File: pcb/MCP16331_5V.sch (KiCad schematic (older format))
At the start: 12 parts, among them U8 MCP16331T

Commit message: Fix inductor (old one was no longer available)
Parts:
- L4: footprint Inductors_local:Inductor_Würth_SPC_4818 -> Inductors_local:Inductor_Würth_WE-PD2_4532
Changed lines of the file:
@@
 F 0 "L4" V 6590 3450 50  0000 C CNN
 F 1 "22µ" V 6499 3450 50  0000 C CNN
-F 2 "Inductors_local:Inductor_Würth_SPC_4818" V 6498 3450 50  0001 C CNN
+F 2 "Inductors_local:Inductor_Würth_WE-PD2_4532" V 6498 3450 50  0001 C CNN
 F 3 "http://katalog.we-online.de/pbs/datasheet/744773122.pdf" V 6498 3450 50  0001 C CNN
 F 4 "732-1258-1-ND" H 6400 3450 60  0001 C CNN "Digi-Key Part Number"

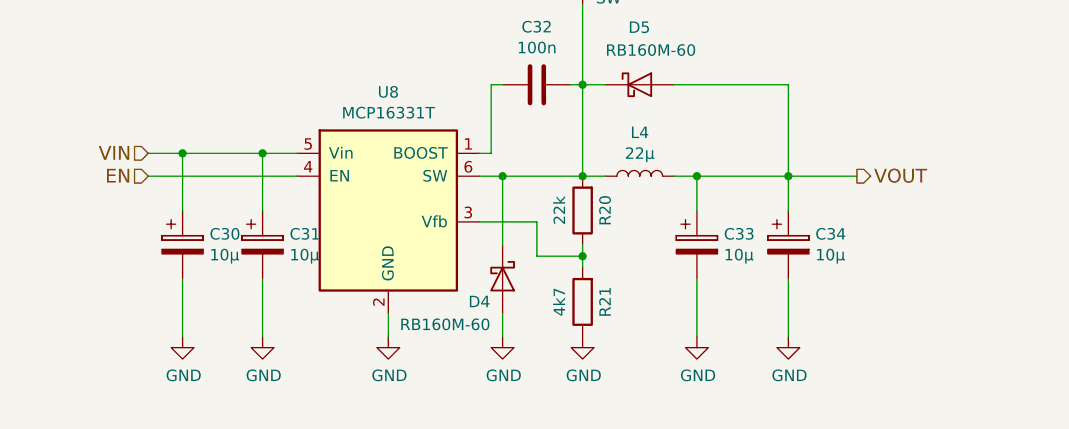
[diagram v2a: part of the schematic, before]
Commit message: Add some improvements, fix issue with schematic error
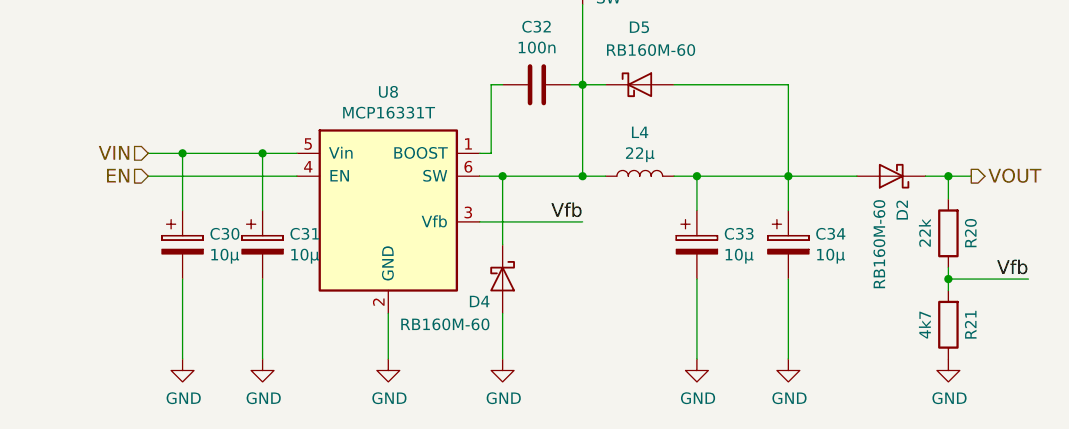
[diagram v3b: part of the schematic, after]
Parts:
- added D2: RB160M-60, Diodes_SMD:SOD-123, symbol D_Schottky
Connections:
- net VOUT: now also R20.2, D2.1 (K); no longer C33.1, C34.1, D5.2 (A), L4.2
- net Vfb: now reaches R20.1, R21.2, U8.3 (Vfb)
- net at C32.2, D4.1 (K), D5.1 (K)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: no longer R20.2
- new net: C33.1, C34.1, D2.2 (A), D5.2 (A), L4.2
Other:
- moved on the sheet: R20, R21
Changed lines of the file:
@@
 LIBS:a4955glptr-t
 LIBS:ap2112k-3.3trg1
+LIBS:lm75bd
+LIBS:mechanical
 LIBS:HighPower-Mechaduino-cache
 EELAYER 25 0
@@
 $EndComp
 $Comp
-L GND #PWR088
+L GND #PWR092
 U 1 1 580BA37A
-P 5300 4150
-F 0 "#PWR088" H 5300 3900 50  0001 C CNN
-F 1 "GND" H 5305 3977 50  0000 C CNN
-F 2 "" H 5300 4150 50  0000 C CNN
-F 3 "" H 5300 4150 50  0000 C CNN
-	1    5300 4150
-	1    0    0    -1
-$EndComp
-Wire Wire Line
-	5300 4050 5300 4150
+P 5300 4250
+F 0 "#PWR092" H 5300 4000 50  0001 C CNN
+F 1 "GND" H 5305 4077 50  0000 C CNN
+F 2 "" H 5300 4250 50  0000 C CNN
+F 3 "" H 5300 4250 50  0000 C CNN
+	1    5300 4250
+	1    0    0    -1
+$EndComp
+Wire Wire Line
+	5300 4050 5300 4250
 $Comp
 L CP C31
@@
 $EndComp
 $Comp
-L GND #PWR089
+L GND #PWR093
 U 1 1 580BA3A1
-P 4750 4150
-F 0 "#PWR089" H 4750 3900 50  0001 C CNN
-F 1 "GND" H 4755 3977 50  0000 C CNN
-F 2 "" H 4750 4150 50  0000 C CNN
-F 3 "" H 4750 4150 50  0000 C CNN
-	1    4750 4150
-	1    0    0    -1
-$EndComp
-$Comp
-L GND #PWR090
+P 4750 4250
+F 0 "#PWR093" H 4750 4000 50  0001 C CNN
+F 1 "GND" H 4755 4077 50  0000 C CNN
+F 2 "" H 4750 4250 50  0000 C CNN
+F 3 "" H 4750 4250 50  0000 C CNN
+	1    4750 4250
+	1    0    0    -1
+$EndComp
+$Comp
+L GND #PWR094
 U 1 1 580BA3A7
-P 4400 4150
-F 0 "#PWR090" H 4400 3900 50  0001 C CNN
-F 1 "GND" H 4405 3977 50  0000 C CNN
-F 2 "" H 4400 4150 50  0000 C CNN
-F 3 "" H 4400 4150 50  0000 C CNN
-	1    4400 4150
-	1    0    0    -1
-$EndComp
-Wire Wire Line
-	4750 3900 4750 4150
-Wire Wire Line
-	4400 3900 4400 4150
+P 4400 4250
+F 0 "#PWR094" H 4400 4000 50  0001 C CNN
+F 1 "GND" H 4405 4077 50  0000 C CNN
+F 2 "" H 4400 4250 50  0000 C CNN
+F 3 "" H 4400 4250 50  0000 C CNN
+	1    4400 4250
+	1    0    0    -1
+$EndComp
+Wire Wire Line
+	4750 3900 4750 4250
+Wire Wire Line
+	4400 3900 4400 4250
 $Comp
 L C C32
@@
 $EndComp
 $Comp
-L GND #PWR091
+L GND #PWR095
 U 1 1 580BA3CF
-P 6650 4150
-F 0 "#PWR091" H 6650 3900 50  0001 C CNN
-F 1 "GND" H 6655 3977 50  0000 C CNN
-F 2 "" H 6650 4150 50  0000 C CNN
-F 3 "" H 6650 4150 50  0000 C CNN
-	1    6650 4150
-	1    0    0    -1
-$EndComp
-$Comp
-L GND #PWR092
+P 6650 4250
+F 0 "#PWR095" H 6650 4000 50  0001 C CNN
+F 1 "GND" H 6655 4077 50  0000 C CNN
+F 2 "" H 6650 4250 50  0000 C CNN
+F 3 "" H 6650 4250 50  0000 C CNN
+	1    6650 4250
+	1    0    0    -1
+$EndComp
+$Comp
+L GND #PWR096
 U 1 1 580BA3D5
-P 7050 4150
-F 0 "#PWR092" H 7050 3900 50  0001 C CNN
-F 1 "GND" H 7055 3977 50  0000 C CNN
-F 2 "" H 7050 4150 50  0000 C CNN
-F 3 "" H 7050 4150 50  0000 C CNN
-	1    7050 4150
-	1    0    0    -1
-$EndComp
-Wire Wire Line
-	6650 3900 6650 4150
-Wire Wire Line
-	7050 3900 7050 4150
+P 7050 4250
+F 0 "#PWR096" H 7050 4000 50  0001 C CNN
+F 1 "GND" H 7055 4077 50  0000 C CNN
+F 2 "" H 7050 4250 50  0000 C CNN
+F 3 "" H 7050 4250 50  0000 C CNN
+	1    7050 4250
+	1    0    0    -1
+$EndComp
+Wire Wire Line
+	6650 3900 6650 4250
+Wire Wire Line
+	7050 3900 7050 4250
 $Comp
 L R R20
 U 1 1 580BA3DD
-P 6150 3600
-F 0 "R20" V 6050 3600 50  0000 C CNN
-F 1 "22k" V 6250 3600 50  0000 C CNN
-F 2 "Resistors_SMD:R_0603" V 6080 3600 50  0001 C CNN
-F 3 "" H 6150 3600 50  0000 C CNN
-F 4 "311-22.0KHRCT-ND" H 6150 3600 60  0001 C CNN "Digi-Key Part Number"
-F 5 "1" H 6150 3600 60  0001 C CNN "Digi-Key Minimum Quantity"
-	1    6150 3600
+P 7750 3700
+F 0 "R20" V 7650 3700 50  0000 C CNN
+F 1 "22k" V 7850 3700 50  0000 C CNN
+F 2 "Resistors_SMD:R_0603" V 7680 3700 50  0001 C CNN
+F 3 "" H 7750 3700 50  0000 C CNN
+F 4 "311-22.0KHRCT-ND" H 7750 3700 60  0001 C CNN "Digi-Key Part Number"
+F 5 "1" H 7750 3700 60  0001 C CNN "Digi-Key Minimum Quantity"
+	1    7750 3700
 	-1   0    0    1
 $EndComp
@@
 L R R21
 U 1 1 580BA3E4
-P 6150 4000
-F 0 "R21" V 6050 4000 50  0000 C CNN
-F 1 "4k7" V 6250 4000 50  0000 C CNN
-F 2 "Resistors_SMD:R_0603" V 6080 4000 50  0001 C CNN
-F 3 "" H 6150 4000 50  0000 C CNN
-F 4 "311-4.70KHRCT-ND" H 6150 4000 60  0001 C CNN "Digi-Key Part Number"
-F 5 "1" H 6150 4000 60  0001 C CNN "Digi-Key Minimum Quantity"
-	1    6150 4000
+P 7750 4100
+F 0 "R21" V 7650 4100 50  0000 C CNN
+F 1 "4k7" V 7850 4100 50  0000 C CNN
+F 2 "Resistors_SMD:R_0603" V 7680 4100 50  0001 C CNN
+F 3 "" H 7750 4100 50  0000 C CNN
+F 4 "311-4.70KHRCT-ND" H 7750 4100 60  0001 C CNN "Digi-Key Part Number"
+F 5 "1" H 7750 4100 60  0001 C CNN "Digi-Key Minimum Quantity"
+	1    7750 4100
 	-1   0    0    1
 $EndComp
 $Comp
-L GND #PWR093
+L GND #PWR097
 U 1 1 580BA3EB
-P 6150 4150
-F 0 "#PWR093" H 6150 3900 50  0001 C CNN
-F 1 "GND" H 6155 3977 50  0000 C CNN
-F 2 "" H 6150 4150 50  0000 C CNN
-F 3 "" H 6150 4150 50  0000 C CNN
-	1    6150 4150
-	1    0    0    -1
-$EndComp
-Wire Wire Line
-	6150 3750 6150 3850
-Wire Wire Line
-	5700 3650 5950 3650
-Wire Wire Line
-	5950 3650 5950 3800
-Connection ~ 6150 3800
+P 7750 4250
+F 0 "#PWR097" H 7750 4000 50  0001 C CNN
+F 1 "GND" H 7755 4077 50  0000 C CNN
+F 2 "" H 7750 4250 50  0000 C CNN
+F 3 "" H 7750 4250 50  0000 C CNN
+	1    7750 4250
+	1    0    0    -1
+$EndComp
+Wire Wire Line
+	5700 3650 6150 3650
 $Comp
 L D_Schottky D4
@@
 Connection ~ 5800 3450
 $Comp
-L GND #PWR094
+L GND #PWR098
 U 1 1 580BA3FF
-P 5800 4150
-F 0 "#PWR094" H 5800 3900 50  0001 C CNN
-F 1 "GND" H 5805 3977 50  0000 C CNN
-F 2 "" H 5800 4150 50  0000 C CNN
-F 3 "" H 5800 4150 50  0000 C CNN
-	1    5800 4150
-	1    0    0    -1
-$EndComp
-Wire Wire Line
-	5800 4150 5800 4050
+P 5800 4250
+F 0 "#PWR098" H 5800 4000 50  0001 C CNN
+F 1 "GND" H 5805 4077 50  0000 C CNN
+F 2 "" H 5800 4250 50  0000 C CNN
+F 3 "" H 5800 4250 50  0000 C CNN
+	1    5800 4250
+	1    0    0    -1
+$EndComp
+Wire Wire Line
+	5800 4250 5800 4050
 $Comp
 L D_Schottky D5
@@
 Connection ~ 7050 3450
 Connection ~ 6650 3450
-Text HLabel 7350 3450 2    60   Output ~ 0
+Text HLabel 7850 3450 2    60   Output ~ 0
 VOUT
 Wire Wire Line
@@
 	1    0    0    -1
 $EndComp
-Wire Wire Line
-	5950 3800 6150 3800
 Text Notes 1250 1450 0    60   ~ 12
 CALCULATIONS
@@
 	0    -1   -1   0
 $EndComp
+$Comp
+L D_Schottky D2
+U 1 1 583B1A52
+P 7500 3450
+F 0 "D2" V 7450 3550 50  0000 L CNN
+F 1 "RB160M-60" V 7550 3550 50  0000 L CNN
+F 2 "Diodes_SMD:SOD-123" H 7500 3450 50  0001 C CNN
+F 3 "http://rohmfs.rohm.com/en/products/databook/datasheet/discrete/diode/schottky_barrier/rb160m-60.pdf" H 7500 3450 50  0001 C CNN
+F 4 "RB160M-90DKR-ND" H 7500 3450 60  0001 C CNN "Digi-Key Part Number"
+F 5 "1" H 7500 3450 60  0001 C CNN "Digi-Key Minimum Quantity"
+	1    7500 3450
+	-1   0    0    1
+$EndComp
+Wire Wire Line
+	7850 3450 7650 3450
+Wire Wire Line
+	7750 3550 7750 3450
+Connection ~ 7750 3450
+Wire Wire Line
+	7750 3850 7750 3950
+Wire Wire Line
+	7750 3900 8100 3900
+Connection ~ 7750 3900
+Text Label 6150 3650 2    60   ~ 0
+Vfb
+Text Label 8100 3900 2    60   ~ 0
+Vfb
 $EndSCHEMATC
